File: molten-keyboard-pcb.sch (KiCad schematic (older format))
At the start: 9 parts, among them U1 Elite-C

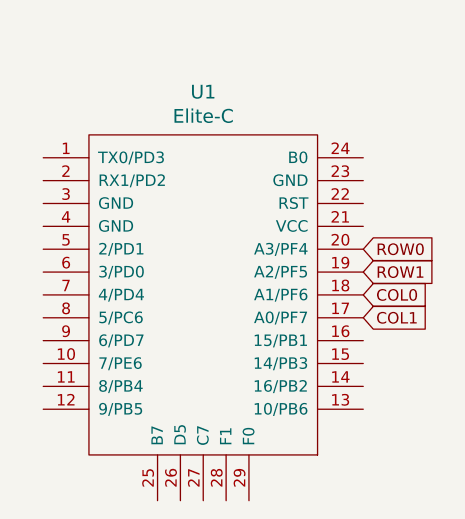
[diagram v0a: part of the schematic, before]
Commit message: Routed tracks
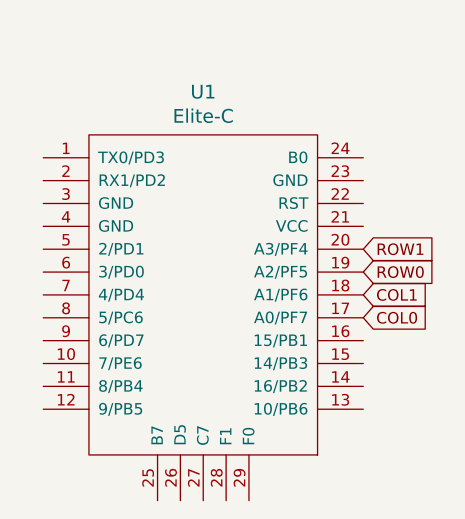
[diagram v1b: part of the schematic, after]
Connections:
- net COL0: now also U1.17 (A0/PF7); no longer U1.18 (A1/PF6)
- net COL1: now also U1.18 (A1/PF6); no longer U1.17 (A0/PF7)
- net ROW0: now also U1.19 (A2/PF5); no longer U1.20 (A3/PF4)
- net ROW1: now also U1.20 (A3/PF4); no longer U1.19 (A2/PF5)
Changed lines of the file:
@@
 Text GLabel 4600 2850 1    50   Input ~ 0
 COL1
+Text GLabel 6600 3750 2    50   Input ~ 0
+ROW0
 Text GLabel 6600 3650 2    50   Input ~ 0
-ROW0
-Text GLabel 6600 3750 2    50   Input ~ 0
 ROW1
+Text GLabel 6600 3950 2    50   Input ~ 0
+COL0
 Text GLabel 6600 3850 2    50   Input ~ 0
-COL0
-Text GLabel 6600 3950 2    50   Input ~ 0
 COL1
 $EndSCHEMATC
